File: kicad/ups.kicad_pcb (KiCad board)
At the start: 2 copper layers, 47 x 47 mm, 64 parts, among them J1 Input, J2 Output, J3 Batt, J4 CE, J5 NTC, J6 2S_MID, Q1 IRF7324, Q2 AO3401A, Q3 AO3401A, Q4 FDS6890A, U1 BQ24610, U2 LM2664M6

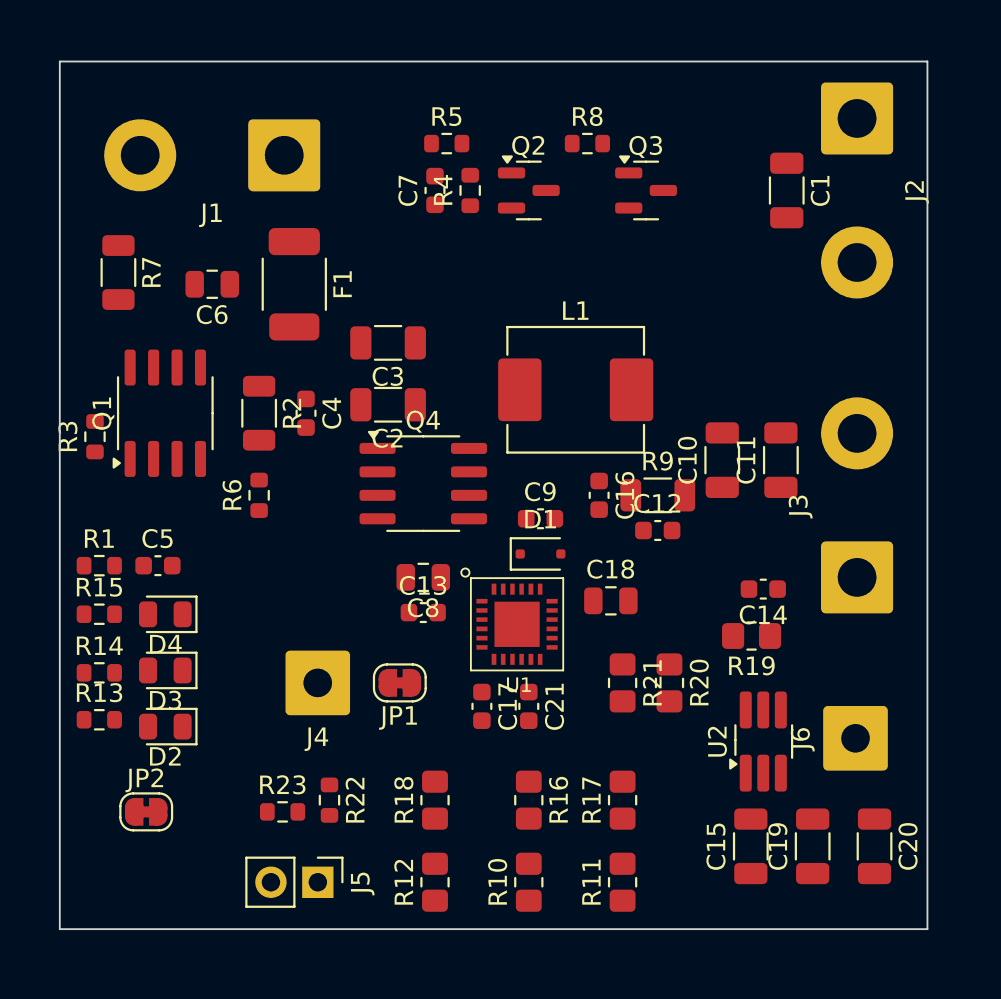
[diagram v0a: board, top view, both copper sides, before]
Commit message: Add PCB and Gerbers
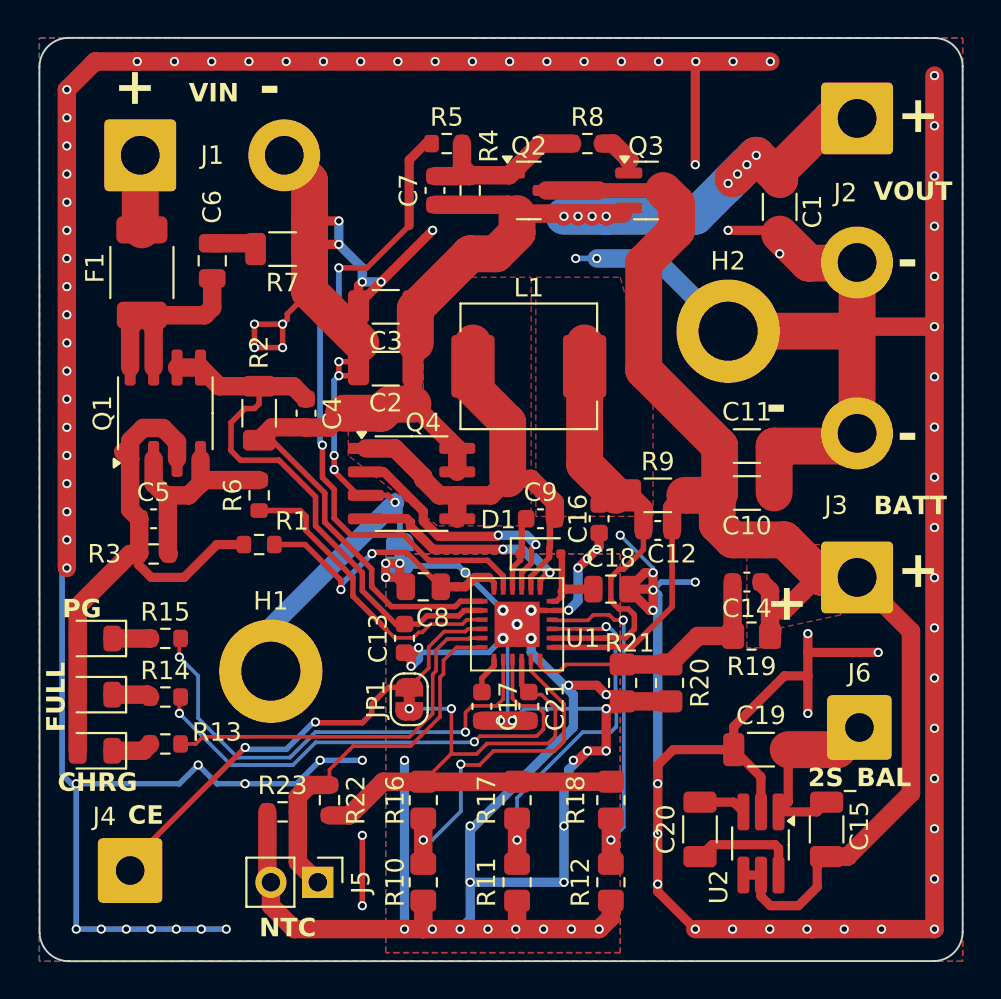
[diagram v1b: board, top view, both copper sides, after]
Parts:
- added H1: MountingHole_Pad, MountingHole:MountingHole_3.2mm_M3_DIN965_Pad, F.Cu at (97.2, 77.5)
- added H2: MountingHole_Pad, MountingHole:MountingHole_3.2mm_M3_DIN965_Pad, F.Cu at (121.9, 59.1)
- F1: value 5A -> Fuse_Small
- J1: value Input -> VIN
- J4: value CE -> Conn_01x01
- JP1: value CE -> SolderJumper_2_Bridged
- JP2: value GND_STAR -> SolderJumper_2_Bridged; moved to B.Cu
- moved JP2 19.6 mm to (104.1, 71.1), turned to -90 degrees
- moved J4 14.4 mm to (89.5, 88.3)
- moved R12 9.52 mm to (115.6, 88.9)
- moved R18 9.52 mm to (115.6, 84.5)
- moved C20 9.50 mm to (120.4, 86.0), turned to 90 degrees
- moved R7 8.98 mm to (97.8, 54.6), turned to 180 degrees
- moved R1 8.73 mm to (96.5, 70.6)
- moved F1 8.28 mm to (90.2, 55.9)
- moved J1 7.80 mm to (90.1, 49.5), turned to 0 degrees
- moved R3 7.10 mm to (90.8, 71.1), turned to 0 degrees
- moved C19 5.94 mm to (123.7, 81.7), turned to 0 degrees
- moved R10 5.72 mm to (105.4, 88.9)
- moved R11 5.72 mm to (110.5, 88.9)
- moved R16 5.72 mm to (105.4, 84.5), turned to 90 degrees
- moved R17 5.72 mm to (110.5, 84.5)
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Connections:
- C5 pad 1: Net-(Q1A-S1) -> Net-(D2-A)
- C9 pad 2: Net-(Q4B-S2) -> Net-(Q4A-S1)
- D2 pad 1: /ST1 -> Net-(D2-K)
- D3 pad 1: /ST2 -> Net-(D3-K)
- D3 pad 2: Net-(D3-A) -> Net-(D2-A)
- D4 pad 1: /PG -> Net-(D4-K)
- D4 pad 2: Net-(D4-A) -> Net-(D2-A)
- L1 pad 1: Net-(Q4B-S2) -> Net-(Q4A-S1)
- Q1 pad 1: Net-(Q1A-S1) -> Net-(D2-A)
- Q1 pad 3: Net-(Q1A-S1) -> Net-(D2-A)
- Q4 pad 1: Earth -> Net-(Q4A-S1)
- Q4 pad 3: Net-(Q4B-S2) -> Earth
- Q4 pad 5: Net-(J2-Pin_1) -> Net-(Q4A-S1)
- Q4 pad 6: Net-(J2-Pin_1) -> Net-(Q4A-S1)
- Q4 pad 7: Net-(Q4B-S2) -> Net-(J2-Pin_1)
- Q4 pad 8: Net-(Q4B-S2) -> Net-(J2-Pin_1)
- R1 pad 1: Net-(Q1A-S1) -> Net-(D2-A)
- R13 pad 1: Net-(Q1A-S1) -> Net-(D2-K)
- R13 pad 2: Net-(D2-A) -> /ST1
- R14 pad 1: Net-(Q1A-S1) -> Net-(D3-K)
- R14 pad 2: Net-(D3-A) -> /ST2
- R15 pad 1: Net-(Q1A-S1) -> Net-(D4-K)
- R15 pad 2: Net-(D4-A) -> /PG
- R3 pad 1: Net-(Q1A-S1) -> Net-(D2-A)
- U1 pad P19: Net-(Q4A-G1) -> Net-(Q4B-G2)
- U1 pad P20: Net-(Q4B-S2) -> Net-(Q4A-S1)
- U1 pad P21: Net-(Q4B-G2) -> Net-(Q4A-G1)
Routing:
- net Earth: track 0.00 -> 343.4 mm, vias 0 -> 104
- net GND: track 0.00 -> 141.4 mm, vias 0 -> 35
- net Net-(J3-Pin_1): track 0.00 -> 86.6 mm
- net Net-(J2-Pin_1): track 0.00 -> 76.2 mm, vias 0 -> 8
- net Net-(U1-~{BATDRV}): track 0.00 -> 35.4 mm, vias 0 -> 2
- net Net-(JP1-A): track 0.00 -> 34.2 mm, vias 0 -> 2
- net Net-(U1-ACP): track 0.00 -> 31.4 mm
- net Net-(D2-A): track 0.00 -> 30.5 mm
- net /ST2: track 0.00 -> 27.6 mm, vias 0 -> 2
- net Net-(Q4A-S1): track 0.00 -> 26.9 mm
- net /PG: track 0.00 -> 26.3 mm, vias 0 -> 2
- net Net-(J4-Pin_1): track 0.00 -> 25.8 mm, vias 0 -> 2
- net Net-(U1-SRP): track 0.00 -> 25.0 mm
- net /ST1: track 0.00 -> 20.6 mm
- net Net-(J5-Pin_1): track 0.00 -> 20.6 mm
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- added copper zone on B.Cu, net Earth
- added copper zone on F.Cu, net Earth
- added copper zone on B.Cu, net GND
- added copper zone on F.Cu, net GND
- added copper zone on F.Cu, net Net-(J3-Pin_1)
- added copper zone on F.Cu, net Net-(Q4A-S1)
- added copper zone on F.Cu, net Net-(U1-SRP)
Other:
- board size 47 x 47 mm -> 50 x 50 mm
- board text added: "+"
- board text added: "-"
- board text added: "2S_BAL"
- board text added: "BATT"
- board text added: "BQ24610 Low Power UPS"
- board text added: "CE"
- board text added: "CHRG"
- board text added: "CONNECT FIRST"
- board text added: "FULL"
- board text added: "NTC"
- board text added: "PG"
- board text added: "VIN"
- board text added: "VOUT"
